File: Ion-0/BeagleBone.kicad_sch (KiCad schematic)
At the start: 3 parts, among them J1 Beaglebone-green-P9, J2 Beaglebone-green-P8

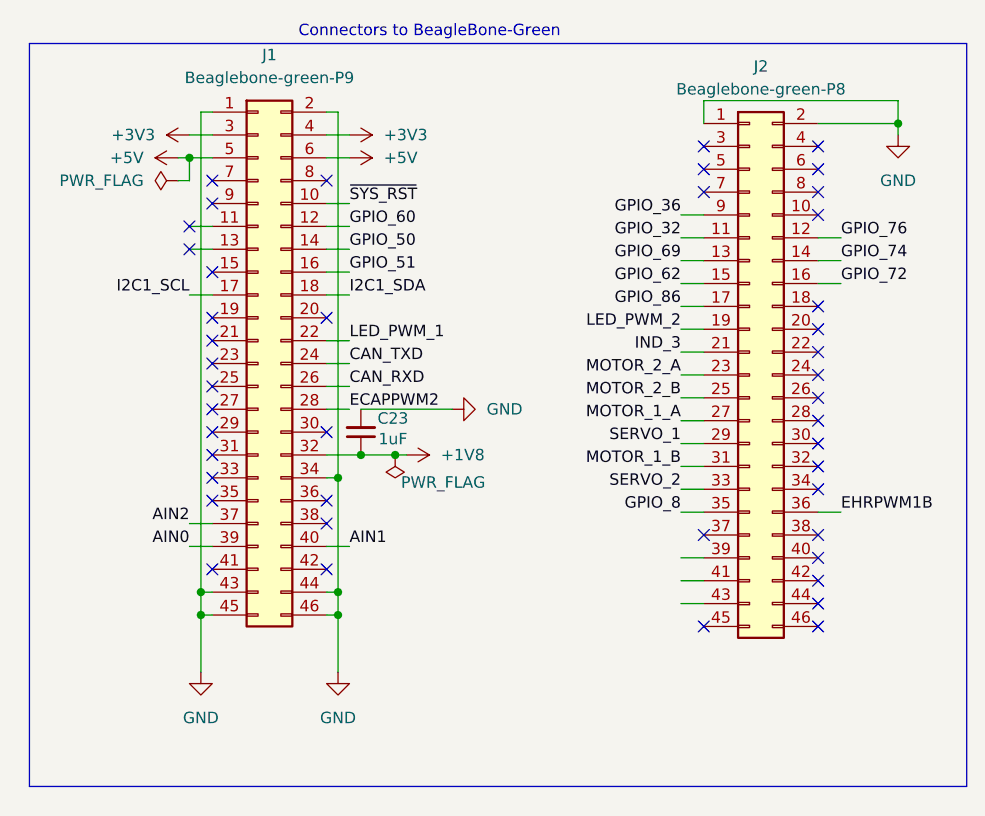
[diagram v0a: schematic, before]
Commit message: fixes in the schematic, made it better
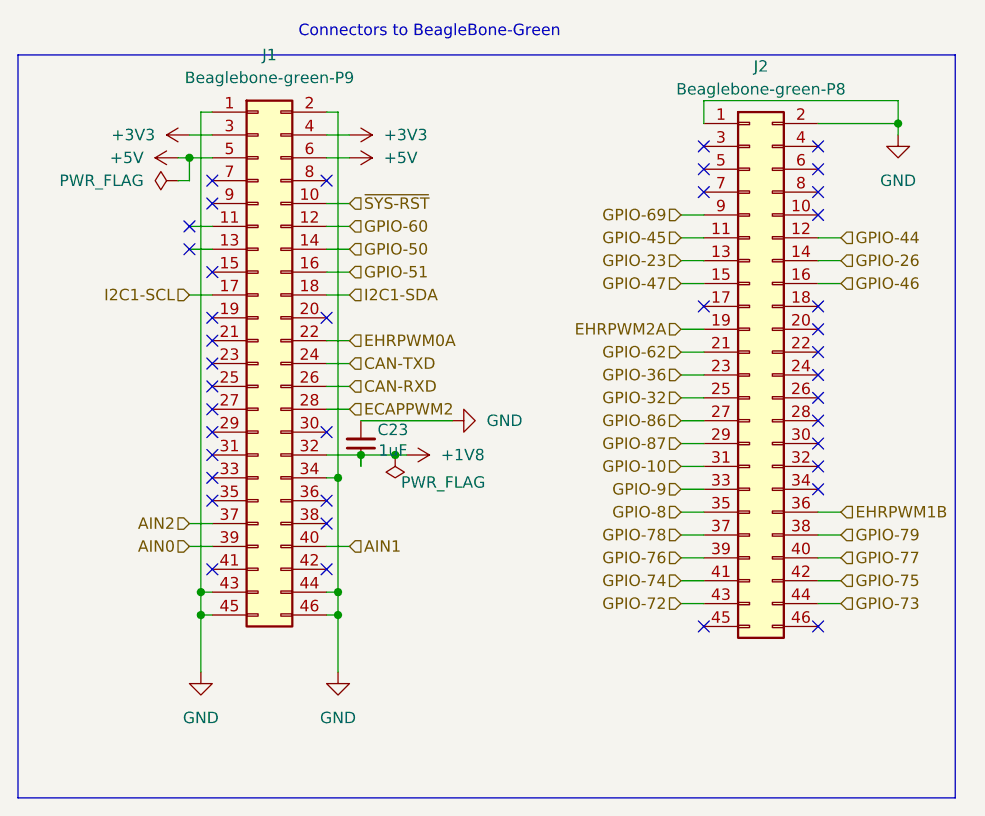
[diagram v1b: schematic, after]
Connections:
- net GPIO-78: now reaches J2.37 (Pin_37)
- net GPIO-79: now reaches J2.38 (Pin_38)
- net GPIO-76: now reaches J2.39 (Pin_39)
- net GPIO-77: now reaches J2.40 (Pin_40)
- net GPIO-74: now reaches J2.41 (Pin_41)
- net GPIO-75: now reaches J2.42 (Pin_42)
- net GPIO-72: now reaches J2.43 (Pin_43)
- net GPIO-73: now reaches J2.44 (Pin_44)
- net CAN_RXD renamed CAN-RXD
- net CAN_TXD renamed CAN-TXD
- net GPIO_32 renamed GPIO-45
- net GPIO_36 renamed GPIO-69
- net GPIO_50 renamed GPIO-50
- net GPIO_51 renamed GPIO-51
- net GPIO_60 renamed GPIO-60
- net GPIO_62 renamed GPIO-47
- net GPIO_69 renamed GPIO-23
- net GPIO_72 renamed GPIO-46
- net GPIO_74 renamed GPIO-26
- net GPIO_76 renamed GPIO-44
- net GPIO_8 renamed GPIO-8
- net GPIO_86: no longer names the net of J2.17 (Pin_17)
- net I2C1_SCL renamed I2C1-SCL
- net I2C1_SDA renamed I2C1-SDA
- net IND_3 renamed GPIO-62
- net LED_PWM_1 renamed EHRPWM0A
- net LED_PWM_2 renamed EHRPWM2A
- net MOTOR_1_A renamed GPIO-86
- net MOTOR_1_B renamed GPIO-10
- net MOTOR_2_A renamed GPIO-36
- net MOTOR_2_B renamed GPIO-32
- net SERVO_1 renamed GPIO-87
- net SERVO_2 renamed GPIO-9
- net ~{SYS_RST} renamed ~{SYS-RST}
- no-connect marks 44 -> 40
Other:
- moved on the sheet: C23
